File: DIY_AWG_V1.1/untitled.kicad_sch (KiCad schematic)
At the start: 89 parts, among them CN1 RH-5019, CN2 RH-5019, CN3 RH-5019, CN4 RH-5019, CN5 RH-5019, J1 Conn_01x04_Socket, U1 AMS1117-3.3, U2 ADP7118ARDZ-3.3-R7, U3 ADP7118ARDZ-3.3-R7, U4 TPS7A3301RGWR, U5 TPS7A4701RGWR, U6 TPS7A3301RGWR, U7 TPS7A4701RGWR

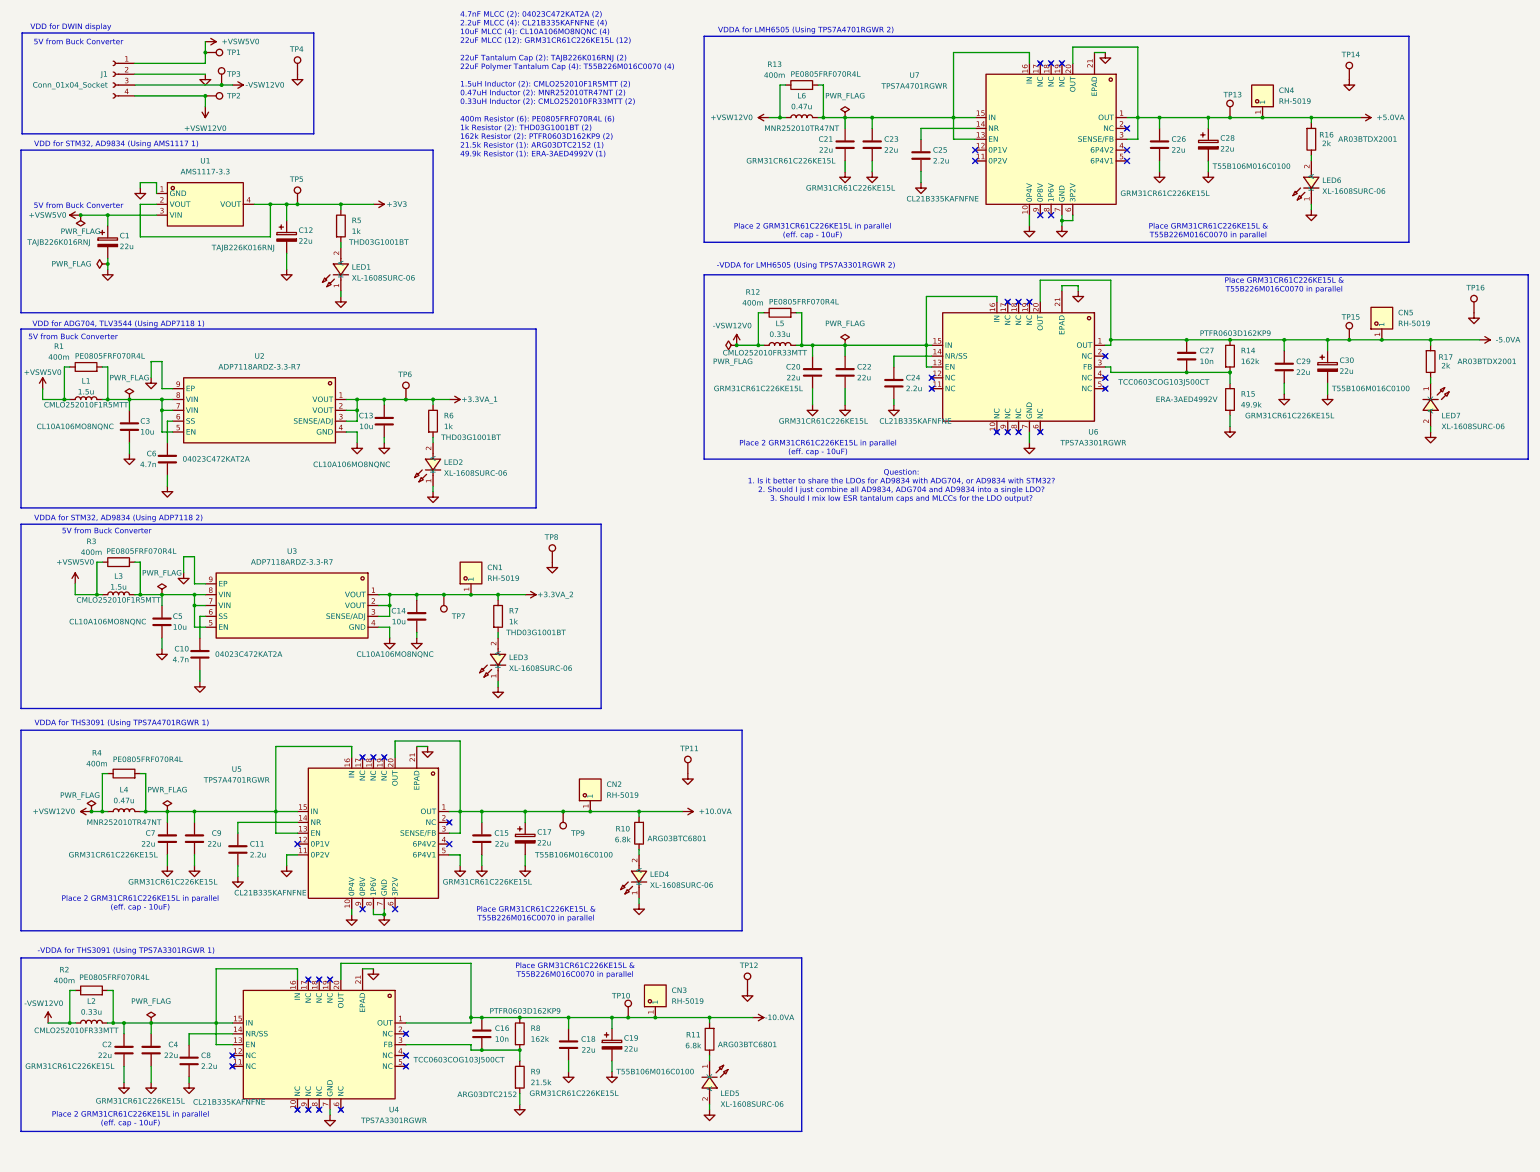
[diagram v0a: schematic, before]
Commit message: Updated PCB schematics
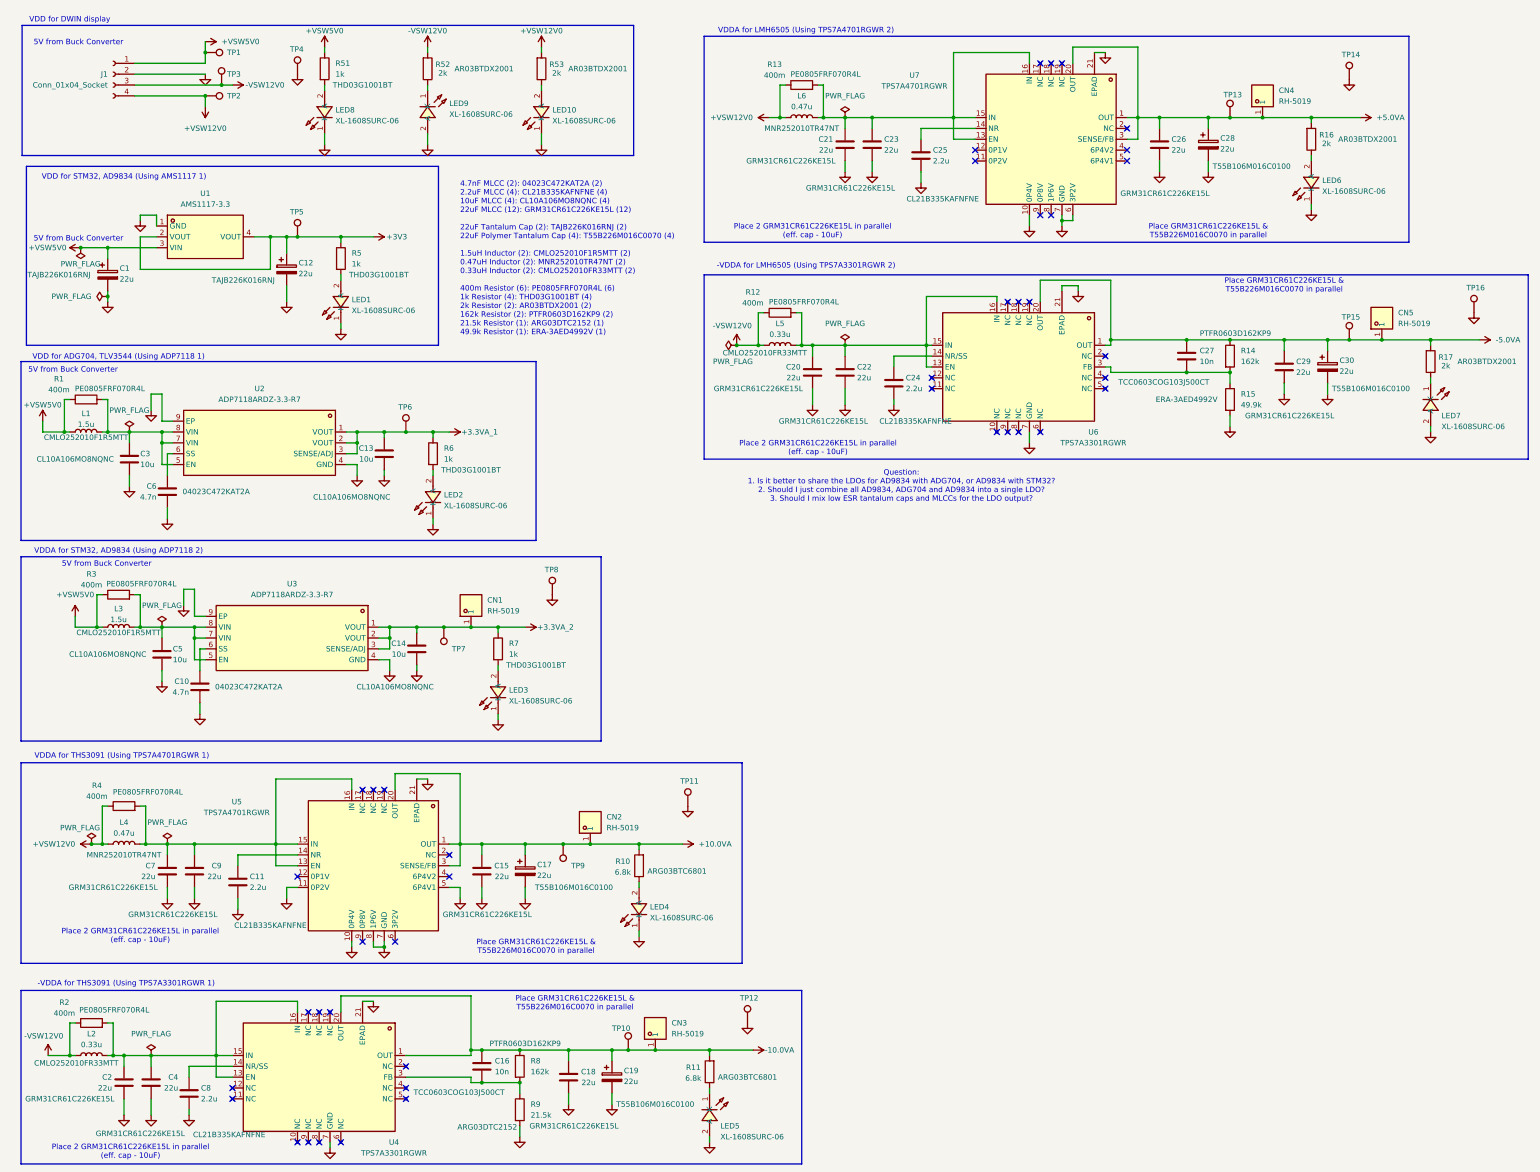
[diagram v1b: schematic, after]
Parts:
- added LED10, LED8, LED9: XL-1608SURC-06, easyeda2kicad:LED0603-RD_RED, symbol easyeda2kicad:XL-1608SURC-06
- added R51: 1k, Resistor_SMD:R_0603_1608Metric, symbol Device:R
- added R52, R53: 2k, Resistor_SMD:R_0603_1608Metric, symbol Device:R
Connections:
- net +VSW12V0: now also R53.2
- net +VSW5V0: now also R51.1
- net -VSW12V0: now also R52.2
- net GND: now also LED10.1 (K), LED8.1 (K), LED9.2 (A)
- new net: LED9.1 (K), R52.1
- new net: LED8.2 (A), R51.2
- new net: LED10.2 (A), R53.1
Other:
- moved on the sheet: C1, C10, C11, C12, C13, C14, C15, C16, C17, C18, C19, C2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
